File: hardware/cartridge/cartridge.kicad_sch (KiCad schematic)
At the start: 31 parts, among them U1 SN74LVC8T245PWR, U2 SN74LVC8T245PWR, U3 SN74LVC8T245PWR, U4 SN74LVC8T245PWR, U5 LCMXO2-1200HC-4TG100C, U6 MX29LV320EBTI-70G, U7 FM28V100-TG, U8 RP2040-Zero

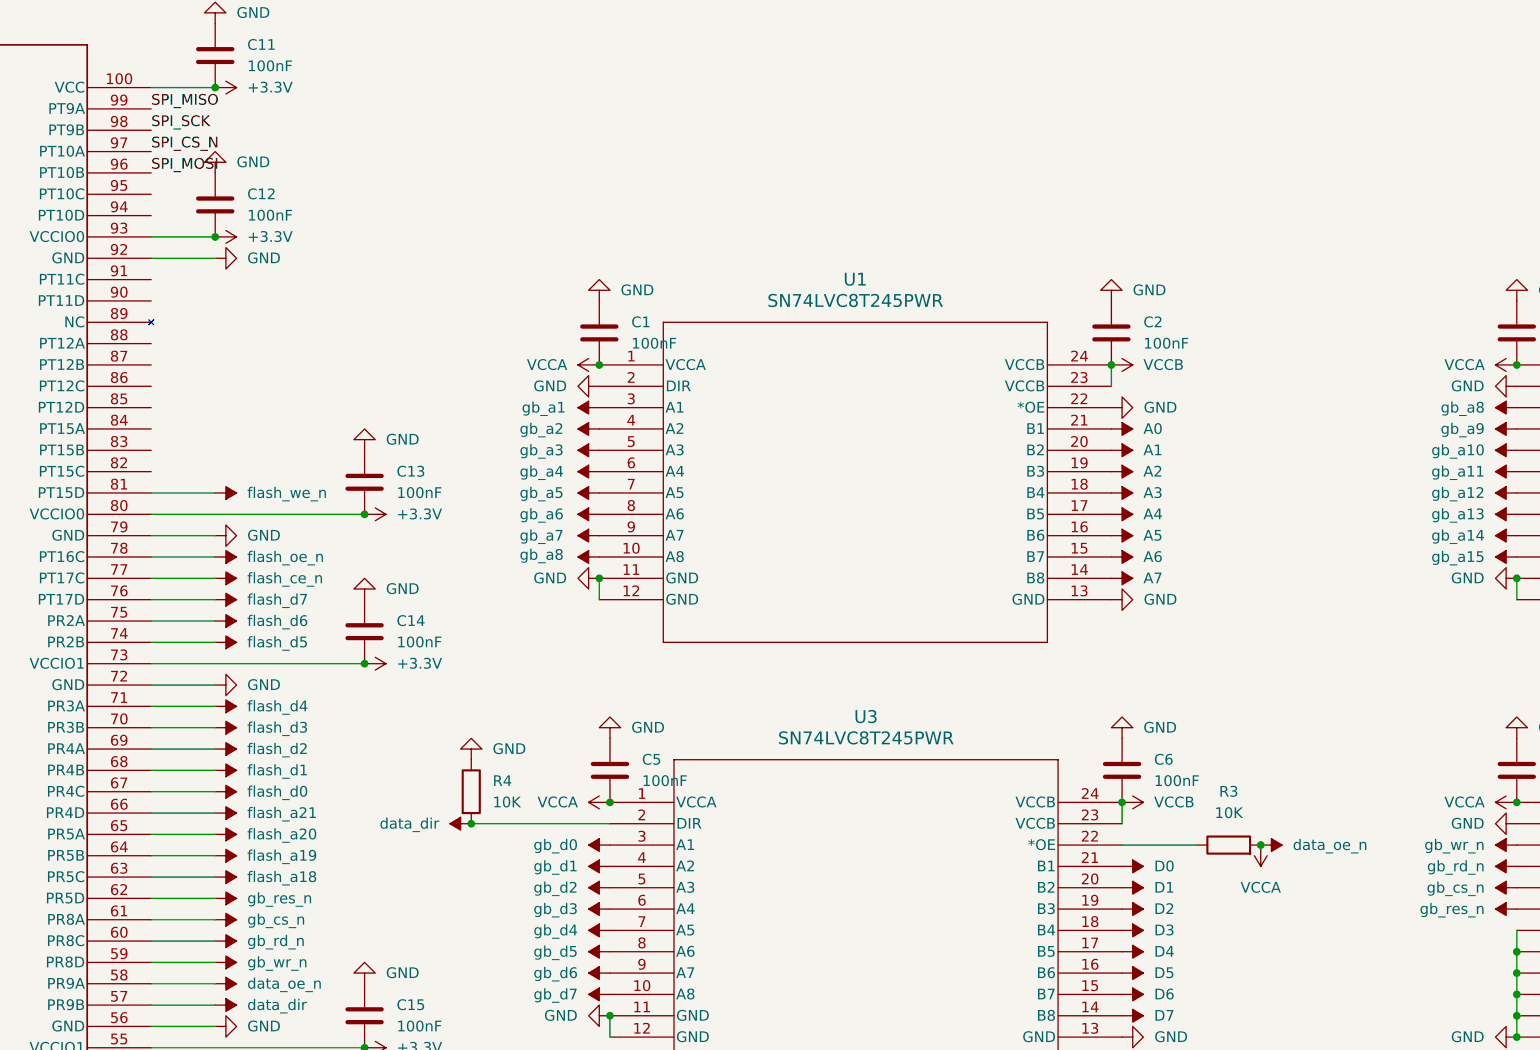
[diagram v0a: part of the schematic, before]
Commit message: Update schematics
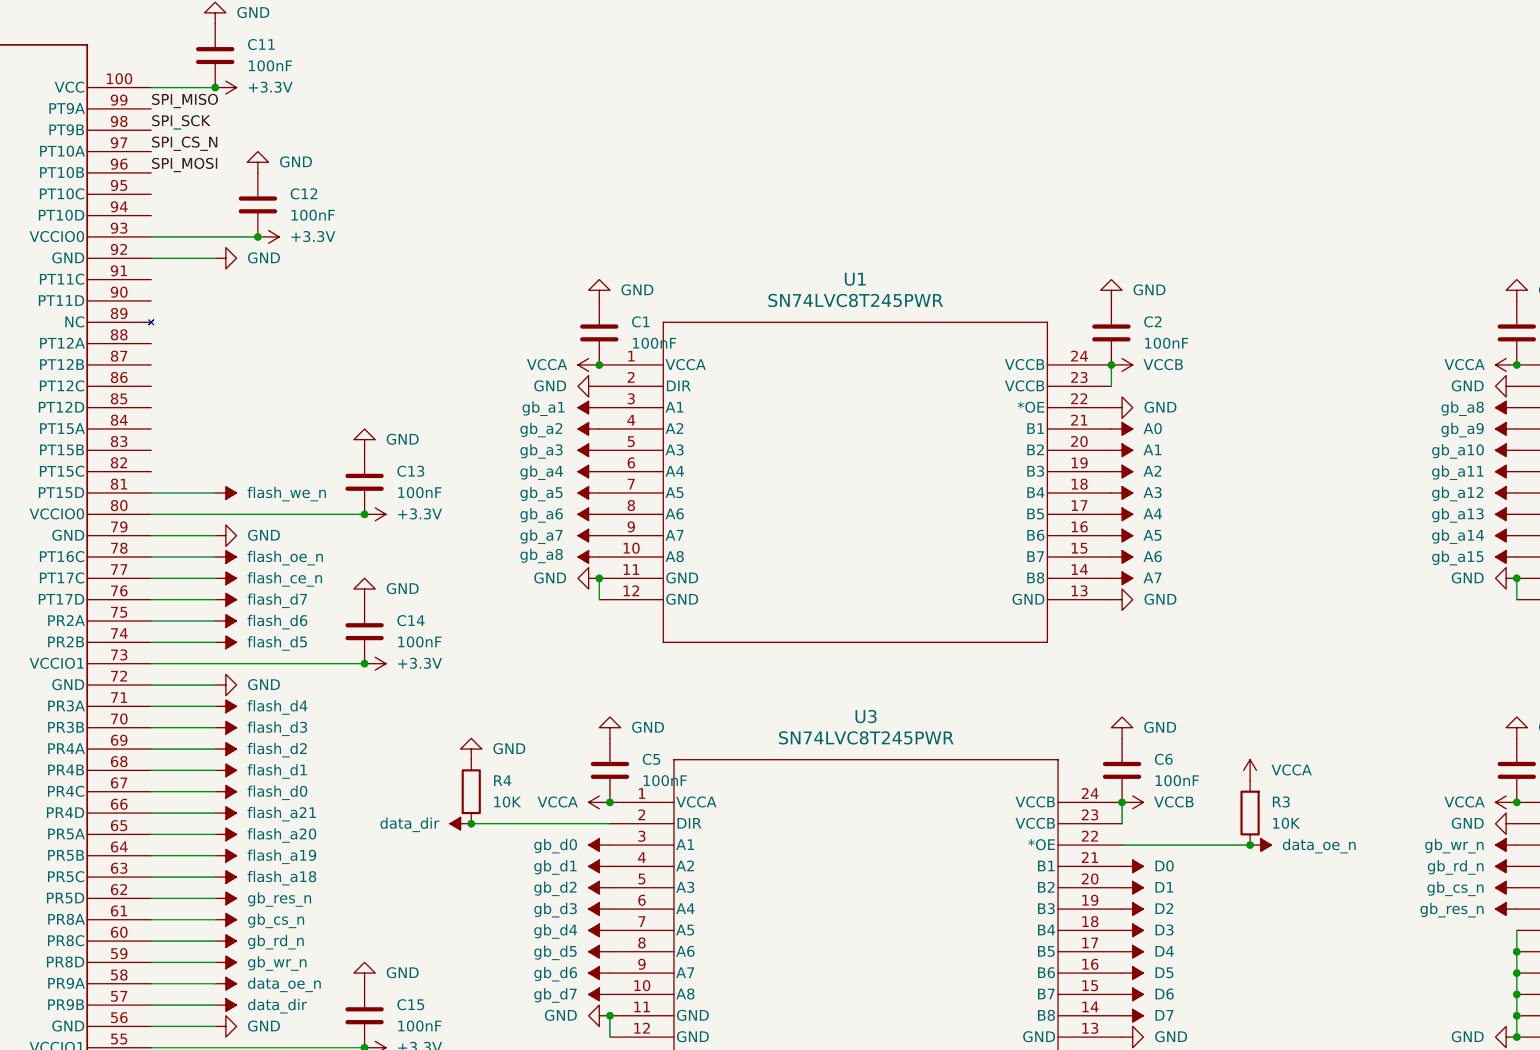
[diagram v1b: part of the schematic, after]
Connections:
- net +3.3V: no longer U5.58 (PR9A)
- net data_oe_n: now reaches R3.1, U3.22 (*OE)
- net data_oe_n: now also U5.58 (PR9A)
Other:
- moved on the sheet: C12
